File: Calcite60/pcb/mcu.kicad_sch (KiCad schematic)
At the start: 10 parts, among them SW2 RESET, U4 E73-2G4M08S1C, Y1 32.768kHz

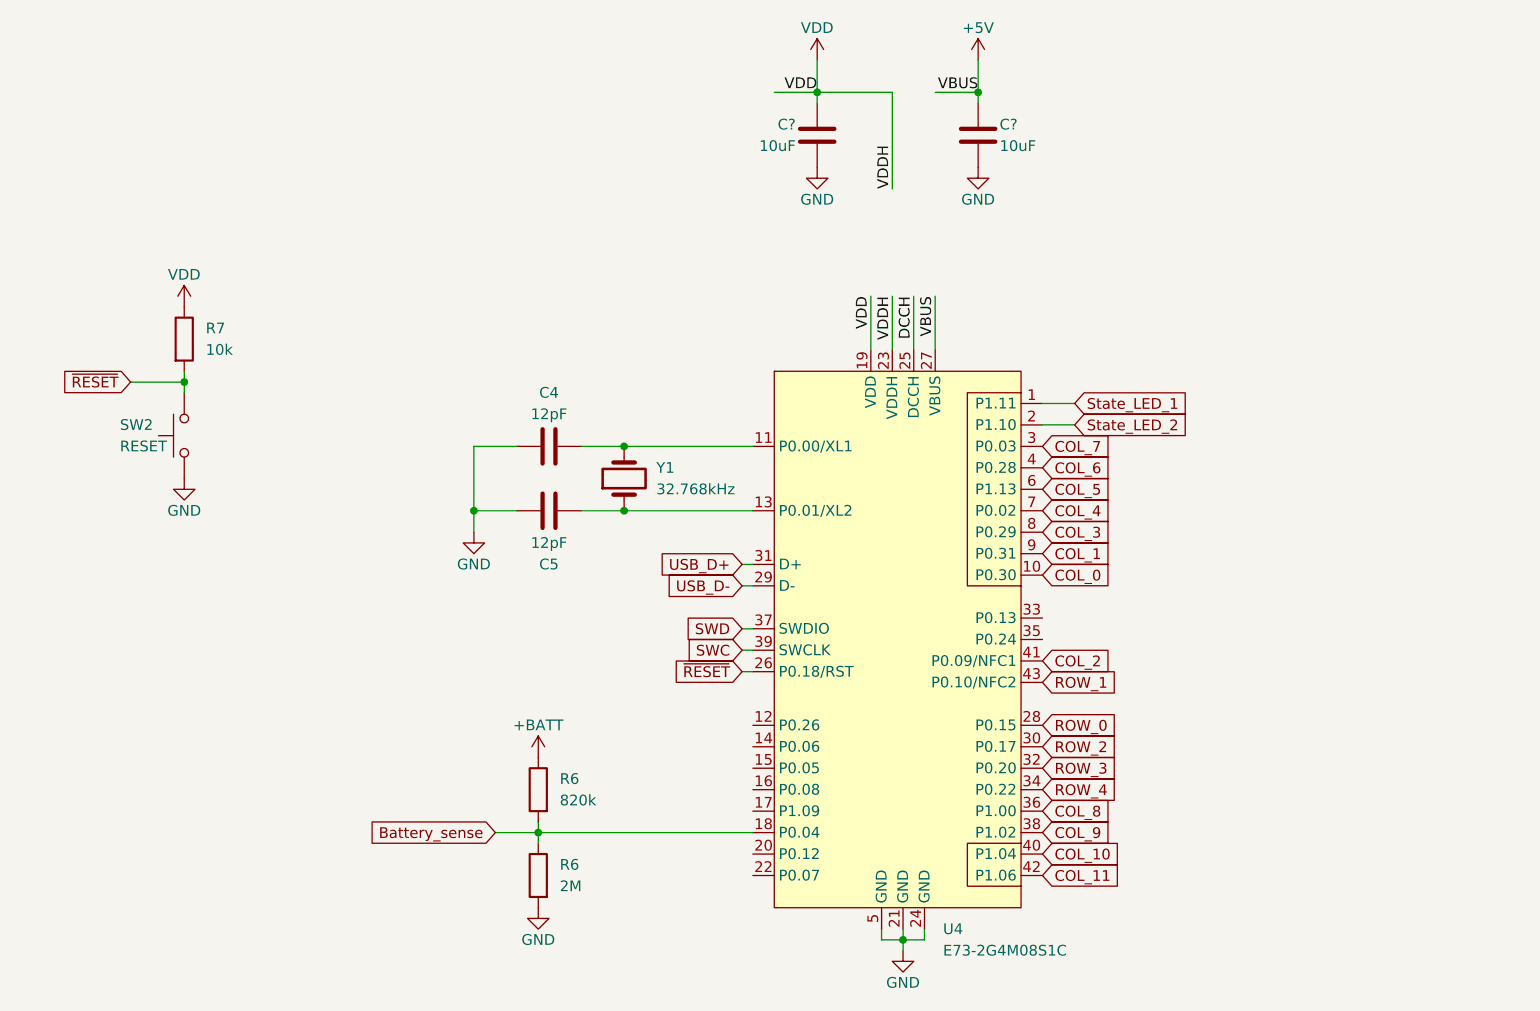
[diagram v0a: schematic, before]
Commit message: Routed
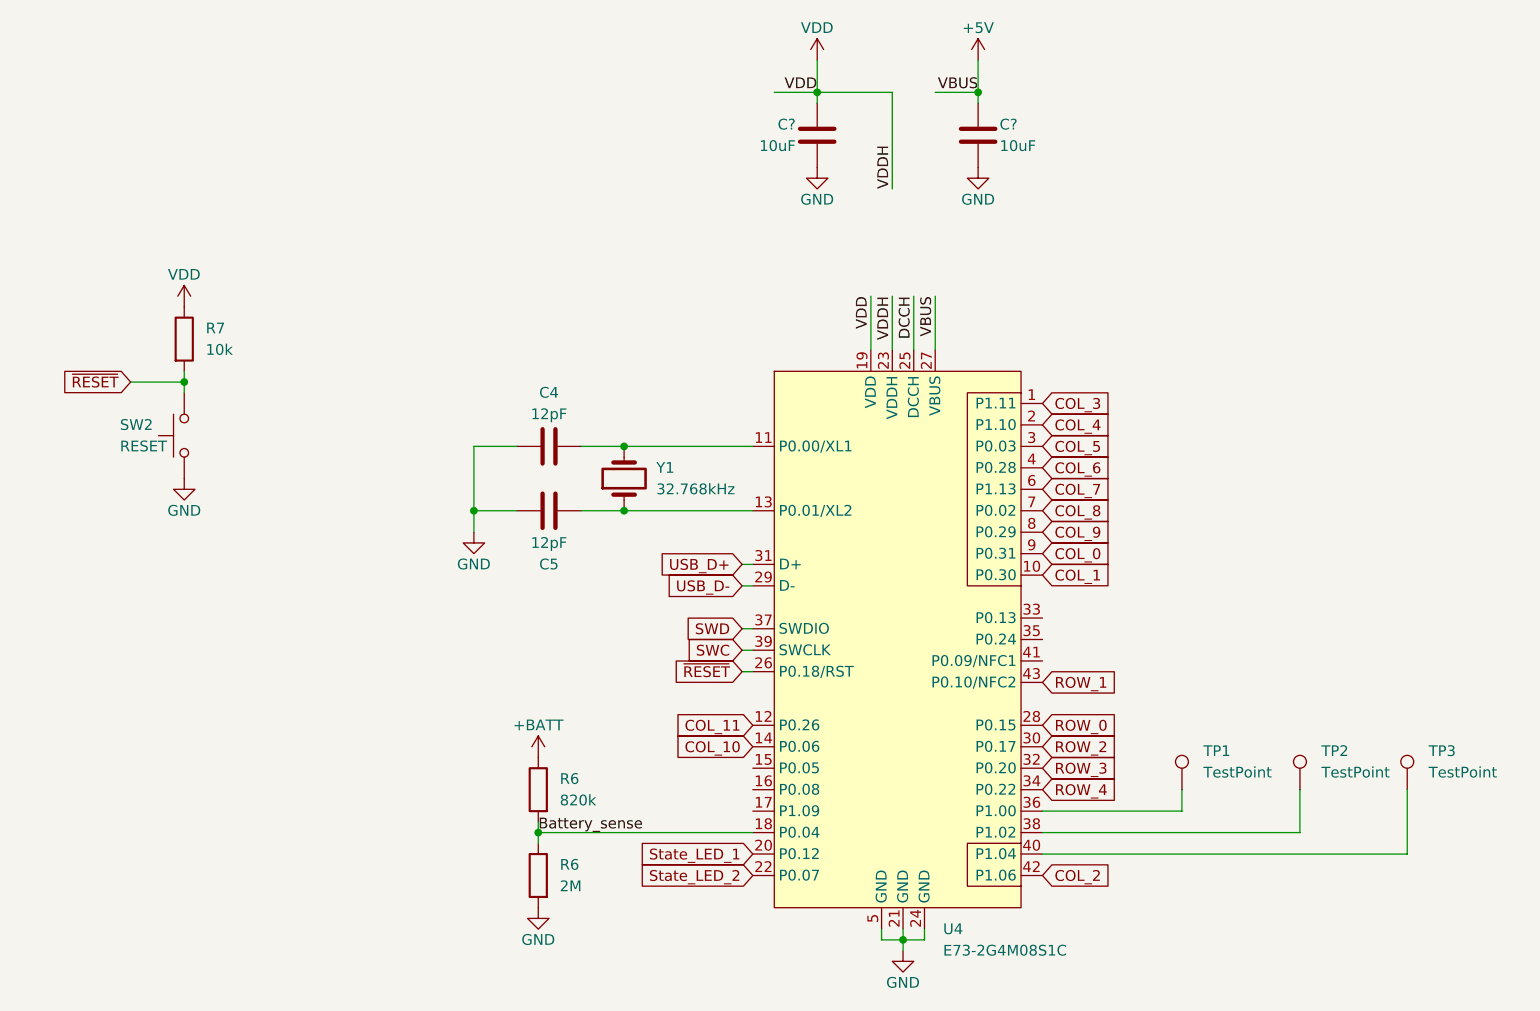
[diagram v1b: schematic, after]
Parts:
- added TP1, TP2, TP3: TestPoint, TestPoint:TestPoint_Pad_D1.5mm, symbol Connector:TestPoint
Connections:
- net COL_0: now also U4.9 (P0.31); no longer U4.10 (P0.30)
- net COL_1: now also U4.10 (P0.30); no longer U4.9 (P0.31)
- net COL_10: now also U4.14 (P0.06); no longer U4.40 (P1.04)
- net COL_11: now also U4.12 (P0.26); no longer U4.42 (P1.06)
- net COL_2: now also U4.42 (P1.06); no longer U4.41 (P0.09/NFC1)
- net COL_3: now also U4.1 (P1.11); no longer U4.8 (P0.29)
- net COL_4: now also U4.2 (P1.10); no longer U4.7 (P0.02)
- net COL_5: now also U4.3 (P0.03); no longer U4.6 (P1.13)
- net COL_7: now also U4.6 (P1.13); no longer U4.3 (P0.03)
- net COL_8: now also U4.7 (P0.02); no longer U4.36 (P1.00)
- net COL_9: now also U4.8 (P0.29); no longer U4.38 (P1.02)
- net State_LED_1: now also U4.20 (P0.12); no longer U4.1 (P1.11)
- net State_LED_2: now also U4.22 (P0.07); no longer U4.2 (P1.10)
- new net: TP1.1, U4.36 (P1.00)
- new net: TP2.1, U4.38 (P1.02)
- new net: TP3.1, U4.40 (P1.04)
